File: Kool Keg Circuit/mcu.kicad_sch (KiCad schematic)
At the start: 40 parts, among them J5 Conn_01x02_Female, J6 Solenoid Conn, 01x02_Male, J7 USB_B_Micro, Q2 2N3906, Q3 BC818, Q4 BC818, SW4 SW_Push, SW5 SW_Push, U5 24LC256-I/MS, U6 946-MPQ6610GS-AEC1-P, U7 CP2102N-Axx-xQFN28, U8 ESP32-WROOM-32D

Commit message: Update footprints, init layout
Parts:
- C15, C16, C17: footprint (none) -> Capacitor_SMD:C_0805_2012Metric_Pad1.18x1.45mm_HandSolder
- C18, C19, C20, C21, C22, C23, C24, C25: footprint Capacitor_SMD:C_0603_1608Metric_Pad1.08x0.95mm_HandSolder -> Capacitor_SMD:C_0805_2012Metric_Pad1.18x1.45mm_HandSolder
- J5: footprint (none) -> Connector_PinHeader_2.00mm:PinHeader_1x04_P2.00mm_Vertical
- J6: footprint (none) -> Connector_Molex:Molex_KK-396_A-41791-0002_1x02_P3.96mm_Vertical
- Q3, Q4: footprint Package_TO_SOT_SMD:SOT-23_Handsoldering -> Package_TO_SOT_SMD:SOT-23_Handsoldering-BC808-25LT1g
- R15, R16, R17: footprint (none) -> Resistor_SMD:R_0805_2012Metric_Pad1.20x1.40mm_HandSolder
- R18, R19, R20, R21, R22, R23, R24, R25, R26: footprint Resistor_SMD:R_0603_1608Metric_Pad0.98x0.95mm_HandSolder -> Resistor_SMD:R_0805_2012Metric_Pad1.20x1.40mm_HandSolder
- SW4, SW5: footprint Button_Switch_SMD:SW_Push_1P1T_NO_6x6mm_H9.5mm -> Button_Switch_THT:KSA_Tactile_SPST
- U5: footprint (none) -> Package_SO:MSOP-8_3x3mm_P0.65mm
- U6: footprint (none) -> Package_SO:SOIC-8_3.9x4.9mm_P1.27mm
- U8: footprint PCB_WORK:PCB_WORK_32D -> RF_Module:ESP32-WROOM-32

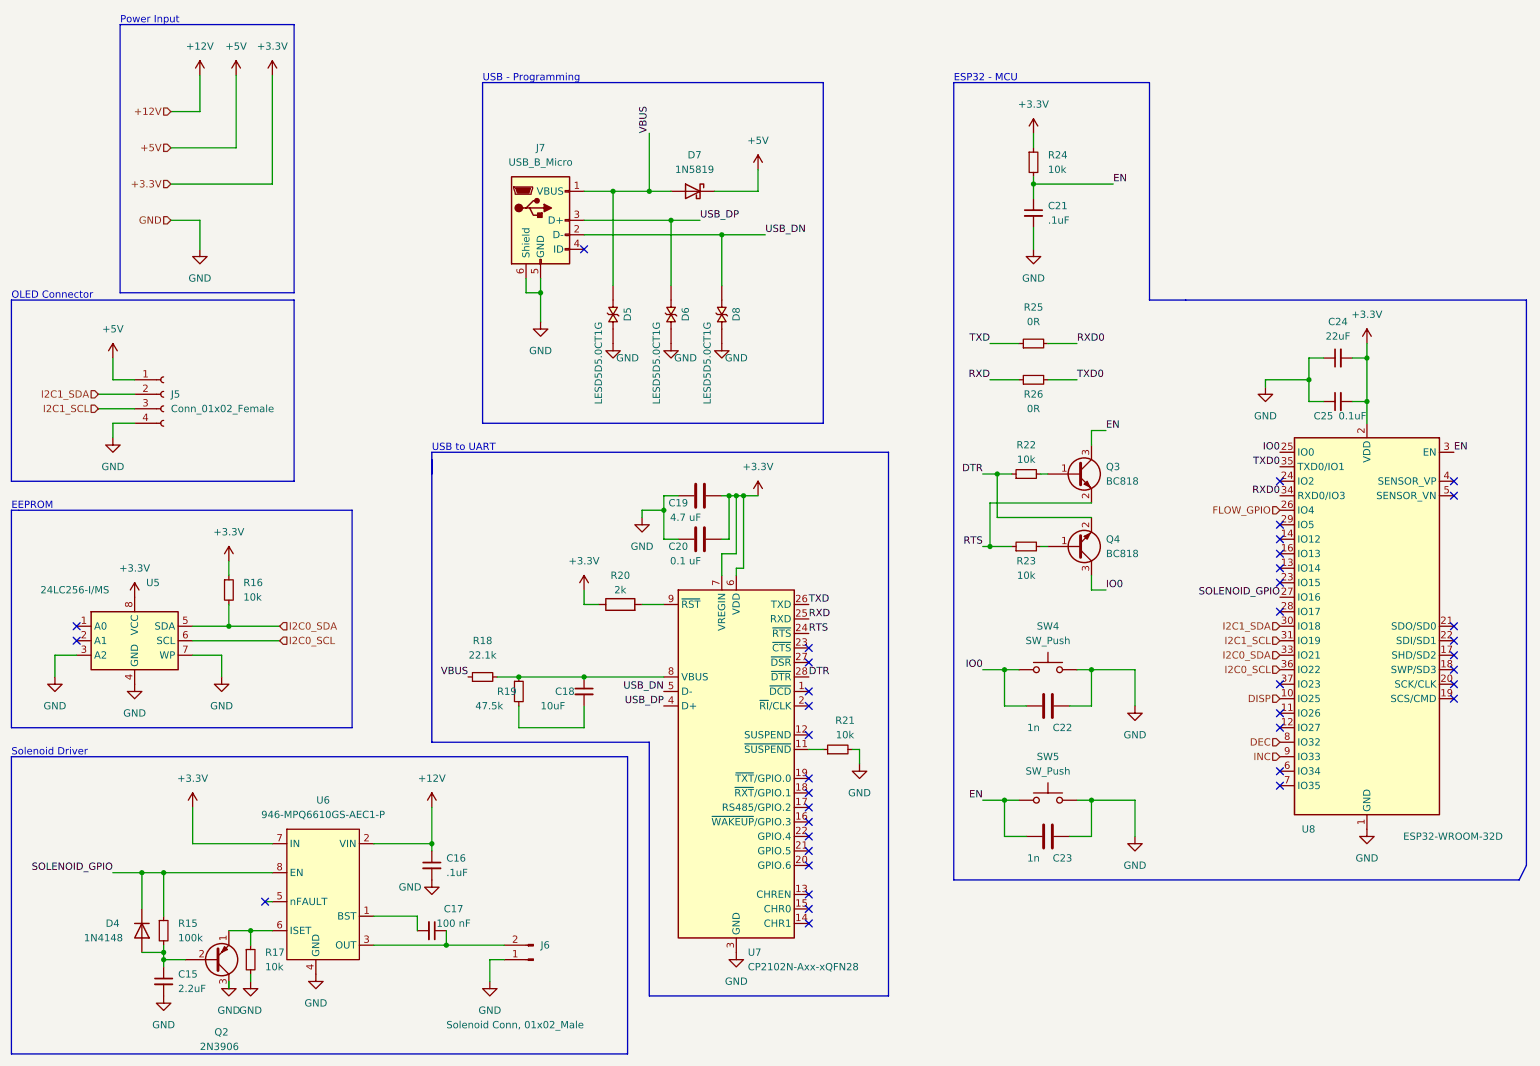
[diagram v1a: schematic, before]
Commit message: PCB
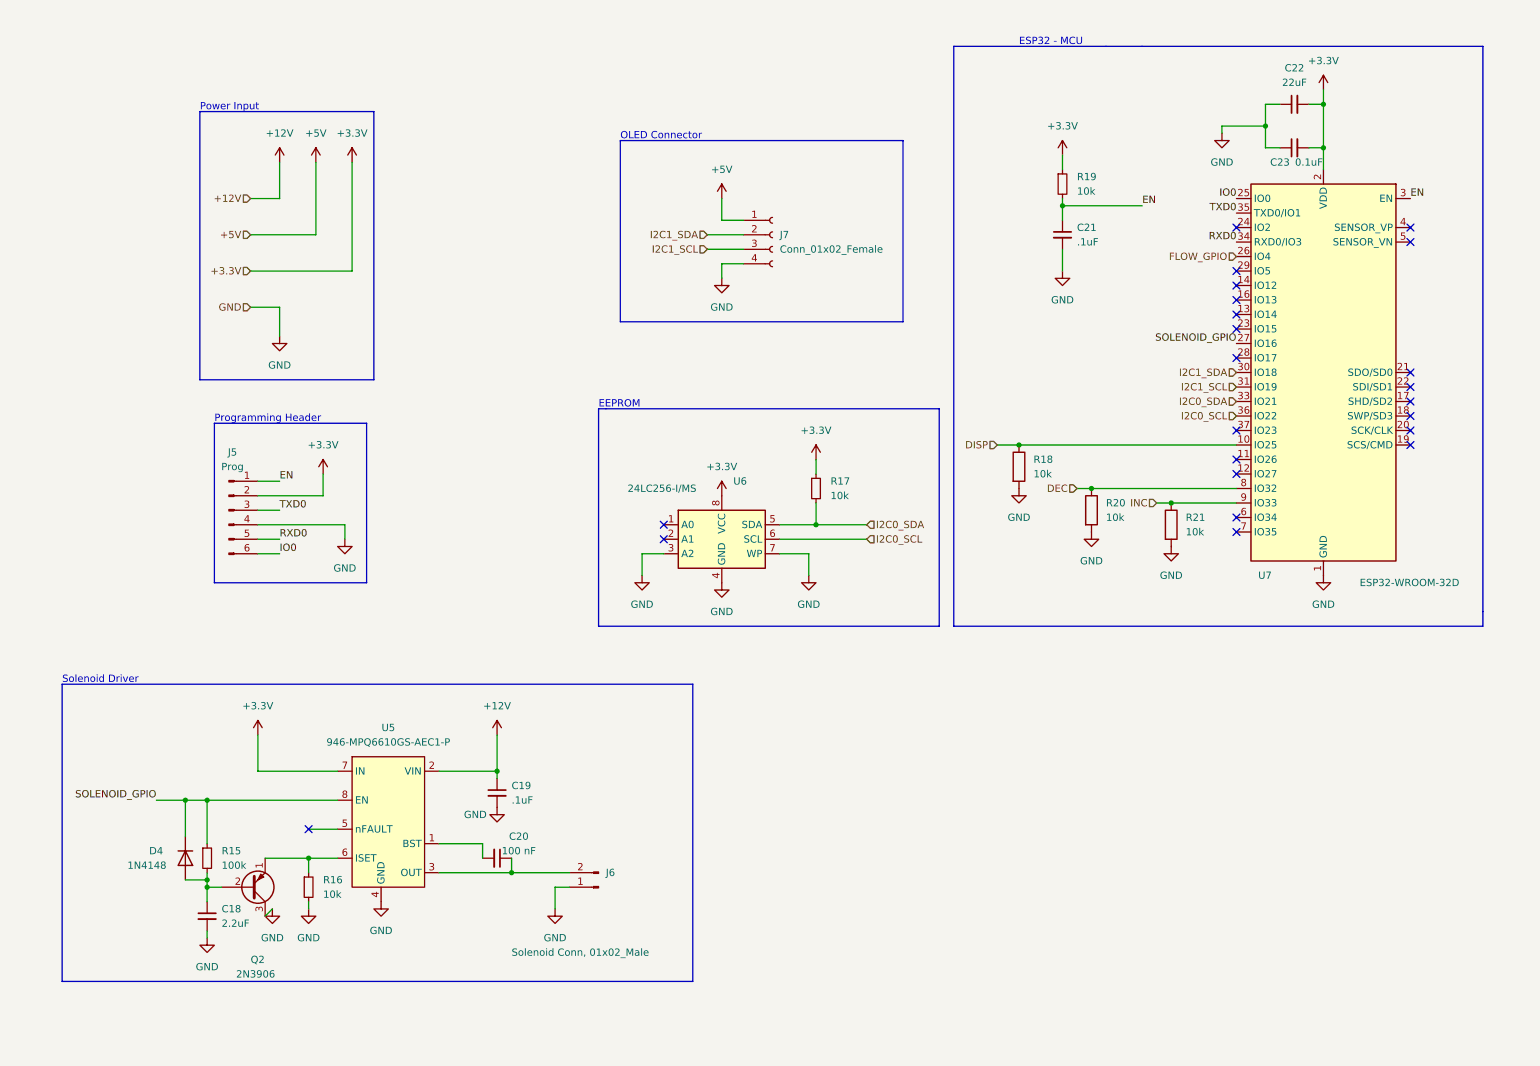
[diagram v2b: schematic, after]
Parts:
- removed C18: 10uF, Capacitor_SMD:C_0805_2012Metric_Pad1.18x1.45mm_HandSolder, symbol Device:C_Small
- removed C19: 4.7 uF, Capacitor_SMD:C_0805_2012Metric_Pad1.18x1.45mm_HandSolder, symbol Device:C
- removed C20: 0.1 uF, Capacitor_SMD:C_0805_2012Metric_Pad1.18x1.45mm_HandSolder, symbol Device:C
- removed C22, C23: 1n, Capacitor_SMD:C_0805_2012Metric_Pad1.18x1.45mm_HandSolder, symbol Device:C
- removed D5, D6, D8: LESD5D5.0CT1G, Diode_SMD:D_SOD-523, symbol LESD5D5.0CT1G:LESD5D5.0CT1G
- removed D7: 1N5819, Diode_SMD:D_1206_3216Metric_Pad1.42x1.75mm_HandSolder, symbol Diode:1N5819
- removed J7: USB_B_Micro, Connector_USB:USB_Micro-B_GCT_USB3076-30-A, symbol Connector:USB_B_Micro
- removed Q3, Q4: BC818, Package_TO_SOT_SMD:SOT-23_Handsoldering-BC808-25LT1g, symbol Transistor_BJT:BC818
- removed R18: 22.1k, Resistor_SMD:R_0805_2012Metric_Pad1.20x1.40mm_HandSolder, symbol Device:R_Small
- removed R19: 47.5k, Resistor_SMD:R_0805_2012Metric_Pad1.20x1.40mm_HandSolder, symbol Device:R_Small
- removed R21, R22, R23: 10k, Resistor_SMD:R_0805_2012Metric_Pad1.20x1.40mm_HandSolder, symbol Device:R_Small
- removed R25, R26: 0R, Resistor_SMD:R_0805_2012Metric_Pad1.20x1.40mm_HandSolder, symbol Device:R_Small
- removed SW4, SW5: SW_Push, Button_Switch_THT:KSA_Tactile_SPST, symbol Switch:SW_Push
- removed U7: CP2102N-Axx-xQFN28, Package_DFN_QFN:QFN-28-1EP_5x5mm_P0.5mm_EP3.35x3.35mm, symbol Interface_USB:CP2102N-Axx-xQFN28
- added J5: Prog, Connector_PinHeader_2.00mm:PinHeader_1x06_P2.00mm_Vertical, symbol Connector:Conn_01x06_Male
- added R18, R21: 10k, Resistor_SMD:R_0805_2012Metric_Pad1.20x1.40mm_HandSolder, symbol Device:R
- R20: value 2k -> 10k
- renumbered C15 to C18, C16 to C19, C17 to C20, C24 to C22, C25 to C23, J5 to J7, R17 to R16, R16 to R17, R24 to R19, U6 to U5, U5 to U6, U8 to U7
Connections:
- net +3.3V: now also J5.2 (Pin_2); no longer R20.1
- net DEC: now also R20.1
- net DISP: now also R18.1
- net EN: now also J5.1 (Pin_1)
- net GND: now also R20.2, J5.4 (Pin_4), R18.2, R21.2
- net INC: now also R21.1
- net IO0: now also J5.6 (Pin_6)
- net RXD0: now also J5.5 (Pin_5)
- net TXD0: now also J5.3 (Pin_3)
- no-connect marks 39 -> 23
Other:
- note added: "Programming Header"
- note removed: "USB - Programming"
- note removed: "USB to UART"
- moved on the sheet: C18, C19, C20, C21, C22, C23, D4, J6, J7, Q2, R15, R16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
